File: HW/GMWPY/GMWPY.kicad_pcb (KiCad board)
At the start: 4 copper layers, 77.6 x 33.4 mm, 63 parts, among them J1 USB_C_Receptacle, J2 Micro_SD_Card_Det, Q1 Q_PJFET_DSG, U1 AMS1117-3.3, U10 LM4040DBZ-2.0, U11 ESP32-S3-WROOM-1, U2 SRV05-4, U3 USEQGCDACH4100, U4 TSV991ILT, U5 TSV991ILT, U6 TSV991ILT, U7 TSV991ILT, U8 TSV991ILT, U9 TSV991ILT

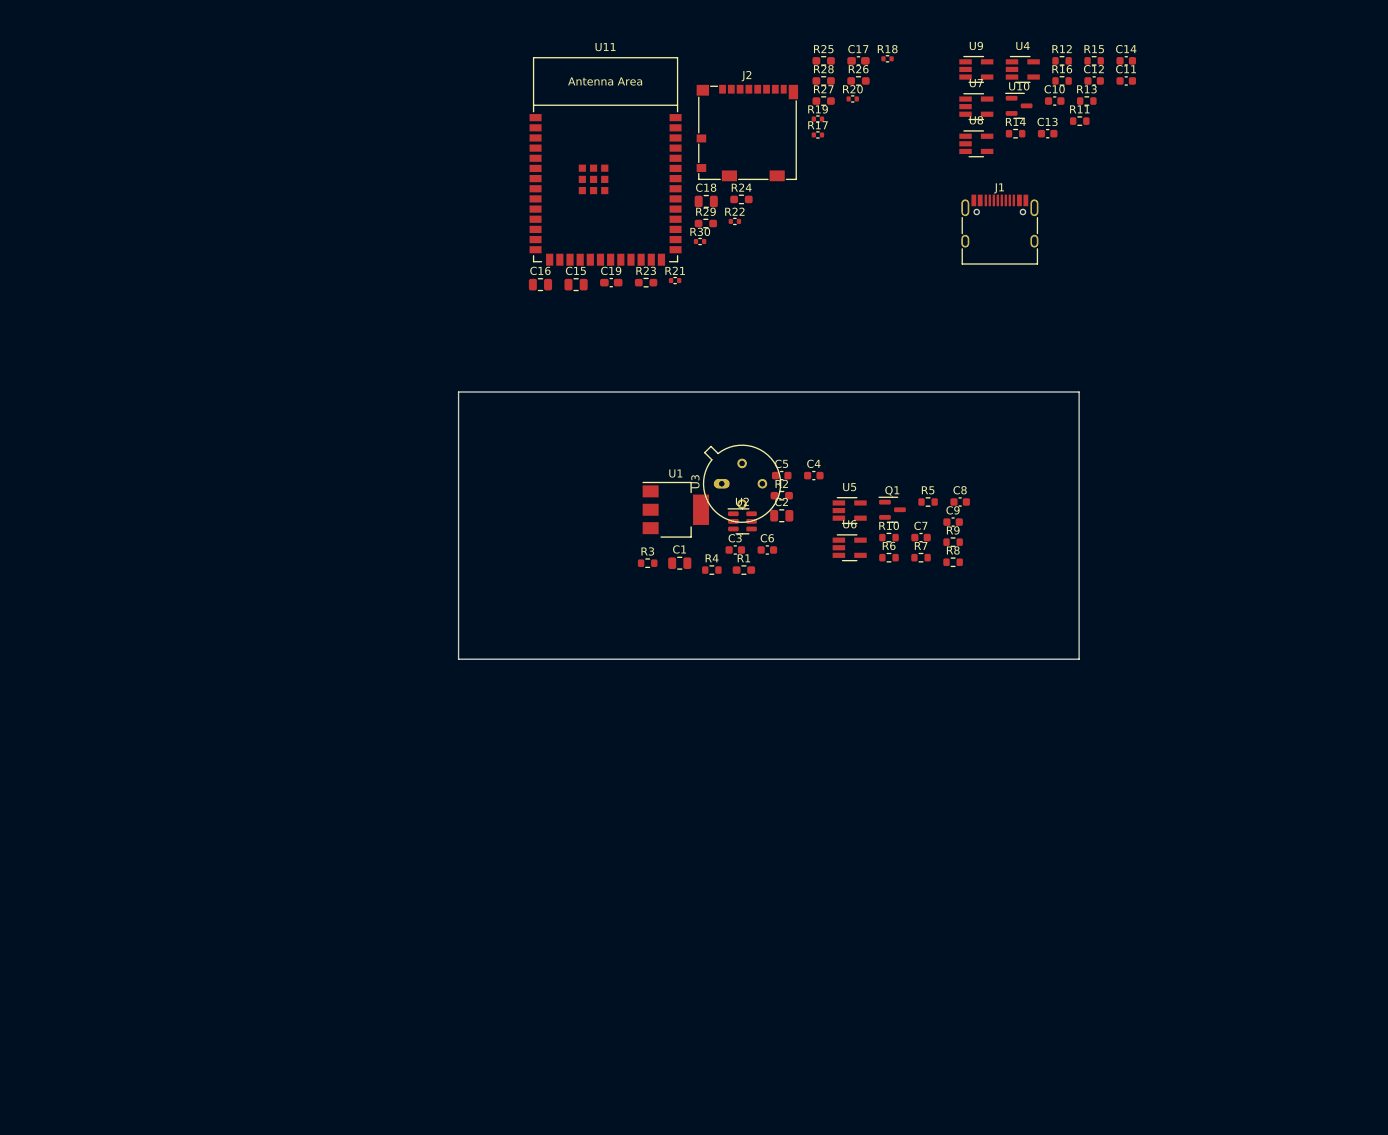
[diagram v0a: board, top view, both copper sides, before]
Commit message: G
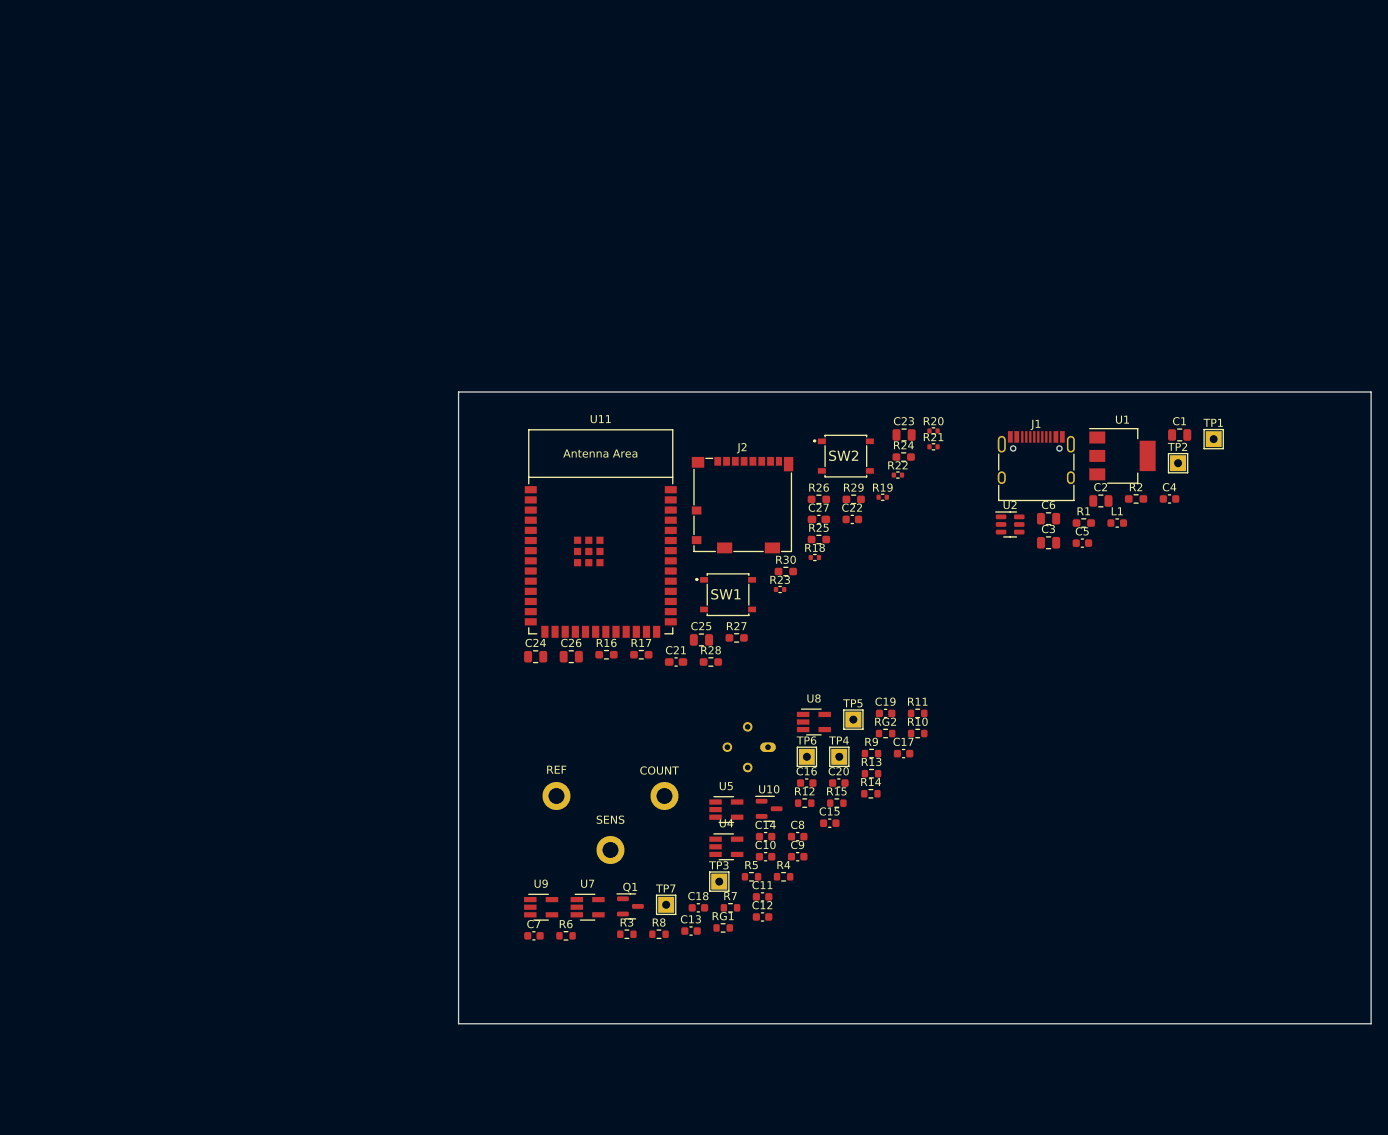
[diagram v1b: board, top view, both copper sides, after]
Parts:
- added C20: 2u2, Capacitor_SMD:C_0603_1608Metric, F.Cu at (131.8, 132.5)
- added C21: 100n, Capacitor_SMD:C_0603_1608Metric_Pad1.08x0.95mm_HandSolder, F.Cu at (111.4, 117.3)
- added C22: 2u2, Capacitor_SMD:C_0603_1608Metric, F.Cu at (133.4, 99.5)
- added C23: 10u, Capacitor_SMD:C_0805_2012Metric, F.Cu at (139.9, 89.0)
- added C24: 10u, Capacitor_SMD:C_0805_2012Metric, F.Cu at (93.9, 116.7)
- added C25: 10u, Capacitor_SMD:C_0805_2012Metric, F.Cu at (114.6, 114.6)
- added C26: 10u, Capacitor_SMD:C_0805_2012Metric, F.Cu at (98.3, 116.7)
- added C27: 100n, Capacitor_SMD:C_0603_1608Metric_Pad1.08x0.95mm_HandSolder, F.Cu at (129.3, 99.5)
- added L1: L_Small, Inductor_SMD:L_0603_1608Metric, F.Cu at (166.6, 100.0)
- added RG1: gain, Resistor_SMD:R_0603_1608Metric, F.Cu at (117.3, 150.6)
- added RG2: gain, Resistor_SMD:R_0603_1608Metric, F.Cu at (137.6, 126.3)
- added SW1: MCU_RESET, SamacSys_Parts:PTS526SK15SMTR2LFS, F.Cu at (117.9, 108.9)
- added SW2: MCU_RESET, SamacSys_Parts:PTS526SK15SMTR2LFS, F.Cu at (132.6, 91.6)
- added TP1: TestPoint, TestPoint:TestPoint_THTPad_2.0x2.0mm_Drill1.0mm, F.Cu at (178.6, 89.5)
- added TP2: TestPoint, TestPoint:TestPoint_THTPad_2.0x2.0mm_Drill1.0mm, F.Cu at (174.2, 92.5)
- added TP3: TestPoint, TestPoint:TestPoint_THTPad_2.0x2.0mm_Drill1.0mm, F.Cu at (116.8, 144.8)
- added TP4: TestPoint, TestPoint:TestPoint_THTPad_2.0x2.0mm_Drill1.0mm, F.Cu at (131.8, 129.2)
- added TP5: TestPoint, TestPoint:TestPoint_THTPad_2.0x2.0mm_Drill1.0mm, F.Cu at (133.6, 124.5)
- added TP6: TestPoint, TestPoint:TestPoint_THTPad_2.0x2.0mm_Drill1.0mm, F.Cu at (127.8, 129.2)
- added TP7: TestPoint, TestPoint:TestPoint_THTPad_2.0x2.0mm_Drill1.0mm, F.Cu at (110.2, 147.7)
- C10, C9: value 100n -> 2u2
- C12, C14: value 2u2 -> 3n3
- C15, C16: value 10u -> 100n; footprint Capacitor_SMD:C_0805_2012Metric -> Capacitor_SMD:C_0603_1608Metric
- C17, C19: value 100n -> 2u2; footprint Capacitor_SMD:C_0603_1608Metric_Pad1.08x0.95mm_HandSolder -> Capacitor_SMD:C_0603_1608Metric
- C18: value 10u -> 2u2; footprint Capacitor_SMD:C_0805_2012Metric -> Capacitor_SMD:C_0603_1608Metric
- C3: value 2u2 -> 10u; footprint Capacitor_SMD:C_0603_1608Metric -> Capacitor_SMD:C_0805_2012Metric
- C6: value 3n3 -> 10u; footprint Capacitor_SMD:C_0603_1608Metric -> Capacitor_SMD:C_0805_2012Metric
- C8: value 3n3 -> 2u2
- R10: value 10k -> 10
- R12: value 10 -> 10k
- R13: value 10k -> 1k
- R16: value 1k -> 10k; footprint Resistor_SMD:R_0603_1608Metric -> Resistor_SMD:R_0603_1608Metric_Pad0.98x0.95mm_HandSolder
- R17, R30: value 10 -> 10k; footprint Resistor_SMD:R_0402_1005Metric -> Resistor_SMD:R_0603_1608Metric_Pad0.98x0.95mm_HandSolder
- R23: value 10k -> 10; footprint Resistor_SMD:R_0603_1608Metric_Pad0.98x0.95mm_HandSolder -> Resistor_SMD:R_0402_1005Metric
- R7: value gain -> 1Meg
- R8: value 1Meg -> 10k
- U3: moved to B.Cu
- U6: value TSV991ILT -> EC4-1000-H2; footprint Package_TO_SOT_SMD:SOT-23-5_HandSoldering -> Z_mycustom_footprint_lib:EC4-3pin; moved to B.Cu
- moved U9 118.0 mm to (94.5, 148.0)
- moved C12 112.4 mm to (122.2, 149.2)
- moved C11 111.7 mm to (122.2, 146.7)
- moved U7 111.2 mm to (100.3, 148.0)
- moved C13 109.2 mm to (113.3, 151.0)
- moved C14 106.9 mm to (122.6, 139.2)
- moved U4 104.0 mm to (117.7, 140.4)
- moved C10 101.1 mm to (122.6, 141.7)
- moved R12 98.2 mm to (127.5, 135.0)
- moved R15 98.2 mm to (131.5, 135.0)
- moved U10 93.3 mm to (123.0, 135.7)
- moved R16 91.6 mm to (102.7, 116.4)
- moved C18 88.3 mm to (114.2, 148.1)
- moved R13 88.3 mm to (135.8, 131.3)
- moved C17 86.8 mm to (139.8, 128.8)
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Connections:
- net /Measurements/Gas renamed /GAS_Measurements/CH4_Gas
- net /Measurements/Ref renamed /GAS_Measurements/CH4_Ref
- C1 pad 1: +5V -> Net-(C1-Pad1)
- C10 pad 1: Net-(C10-Pad1) -> GND
- C10 pad 2: Net-(C10-Pad2) -> +5V
- C11 pad 2: +5V -> Net-(C11-Pad2)
- C12 pad 1: GND -> /GAS_Measurements/OUT2
- C12 pad 2: +5V -> /GAS_Measurements/CH4_V-ref
- C13 pad 2: +5V -> Net-(C13-Pad2)
- C14 pad 1: GND -> /GAS_Measurements/OUT1
- C14 pad 2: Net-(C14-Pad2) -> /GAS_Measurements/CH4_V-gas
- C15 pad 1: +3V3 -> /GAS_Measurements/OUT3
- C15 pad 2: GND -> /GAS_Measurements/H2_V-
- C16 pad 1: +3V3 -> /GAS_Measurements/H2_counter
- C16 pad 2: GND -> Net-(C16-Pad2)
- C17 pad 1: +3V3 -> GND
- C17 pad 2: GND -> +5V
- C18 pad 1: +3V3 -> GND
- C18 pad 2: GND -> +5V
- C19 pad 1: +3V3 -> GND
- C19 pad 2: GND -> +5V
- C3 pad 1: GND -> Net-(C1-Pad1)
- C3 pad 2: +5V -> GND
- C4 pad 2: +5V -> Net-(C1-Pad1)
- C5 pad 2: Net-(C5-Pad2) -> +5V
- C6 pad 1: /Measurements/OUT2 -> +5V
- C6 pad 2: /Measurements/V-ref -> GND
- C7 pad 2: Net-(C7-Pad2) -> +5V
- C8 pad 1: /Measurements/OUT1 -> GND
- C8 pad 2: /Measurements/V-gas -> +5V
- C9 pad 1: /Measurements/OUT3 -> GND
- C9 pad 2: Net-(C9-Pad2) -> +5V
- J2 pad 10: /MCU/CARD_DETECT -> GPIO_40
- Q1 pad 1: Net-(Q1-Pad1) -> /GAS_Measurements/H2_reference
- Q1 pad 2: Net-(Q1-Pad2) -> /GAS_Measurements/H2_sensing
- R10 pad 1: Net-(Q1-Pad1) -> /GAS_Measurements/H2_V-
- R10 pad 2: Net-(C10-Pad2) -> /GAS_Measurements/H2_sensing
- R11 pad 1: Net-(C9-Pad2) -> REF
- R11 pad 2: Net-(Q1-Pad2) -> /GAS_Measurements/H2_V+
- R12 pad 1: REF -> Net-(R12-Pad1)
- R12 pad 2: Net-(R12-Pad2) -> REF
- R13 pad 1: Net-(R13-Pad1) -> +5V
- R13 pad 2: REF -> 2V048
- R14 pad 1: +5V -> /GAS_Measurements/1V012
- R14 pad 2: Net-(C14-Pad2) -> 2V048
- R15 pad 1: Net-(R15-Pad1) -> /GAS_Measurements/1V012
- R15 pad 2: Net-(C14-Pad2) -> GND
- R16 pad 1: Net-(R15-Pad1) -> +3V3
- R16 pad 2: GND -> /MCU/ESP_EN
- R17 pad 1: /MCU/DATA_0 -> /MCU/ESP_BOOT
- R17 pad 2: GPIO_42 -> +3V3
- R18 pad 1: /MCU/DATA_1 -> /MCU/DATA_0
- R18 pad 2: GPIO_41 -> GPIO_42
- R19 pad 1: /MCU/DATA_2 -> /MCU/DATA_1
- R19 pad 2: GPIO_1 -> GPIO_41
- R20 pad 1: /MCU/DATA_3 -> /MCU/DATA_2
- R20 pad 2: GPIO_2 -> GPIO_1
- R21 pad 1: /MCU/CMD -> /MCU/DATA_3
- R21 pad 2: GPIO_43 -> GPIO_2
- R22 pad 1: /MCU/CLK -> /MCU/CMD
- R22 pad 2: GPIO_44 -> GPIO_43
- R23 pad 1: /MCU/DATA_0 -> /MCU/CLK
- R23 pad 2: +3V3 -> GPIO_44
- R24 pad 1: /MCU/DATA_1 -> /MCU/DATA_0
- R25 pad 1: /MCU/DATA_2 -> /MCU/DATA_1
- R26 pad 1: /MCU/DATA_3 -> /MCU/DATA_2
- R27 pad 1: /MCU/CMD -> /MCU/DATA_3
- R28 pad 1: /MCU/CLK -> /MCU/CMD
- R29 pad 1: /MCU/CARD_DETECT -> /MCU/CLK
- R3 pad 1: Net-(C5-Pad2) -> Net-(C11-Pad2)
- R3 pad 2: /Measurements/V-ref -> /GAS_Measurements/CH4_V-ref
- R30 pad 1: /MCU/CARD_DETECT -> GPIO_40
- R30 pad 2: GPIO_40 -> +3V3
- R4 pad 1: Net-(C7-Pad2) -> Net-(C13-Pad2)
- R4 pad 2: /Measurements/V-gas -> /GAS_Measurements/CH4_V-gas
- R5 pad 1: /Measurements/OUT2 -> /GAS_Measurements/OUT2
- R5 pad 2: /Measurements/V-ref -> /GAS_Measurements/CH4_V-ref
- R6 pad 1: /Measurements/OUT1 -> /GAS_Measurements/OUT1
- R6 pad 2: /Measurements/V-gas -> /GAS_Measurements/CH4_V-gas
- R7 pad 1: /Measurements/OUT3 -> GND
- R7 pad 2: Net-(C9-Pad2) -> Net-(Q1-Pad3)
- R8 pad 1: GND -> Net-(C16-Pad2)
- R8 pad 2: Net-(Q1-Pad3) -> Net-(R8-Pad2)
- R9 pad 1: Net-(C10-Pad2) -> /GAS_Measurements/H2_reference
- R9 pad 2: Net-(R9-Pad2) -> Net-(C16-Pad2)
- U1 pad 3: +5V -> Net-(C1-Pad1)
- U10 pad 1: Net-(C14-Pad2) -> 2V048
- U4 pad 1: /Measurements/OUT2 -> /GAS_Measurements/OUT2
- U4 pad 4: /Measurements/V-ref -> /GAS_Measurements/CH4_V-ref
- U5 pad 1: /Measurements/OUT1 -> /GAS_Measurements/OUT1
- U5 pad 4: /Measurements/V-gas -> /GAS_Measurements/CH4_V-gas
- U6 pad 1: Net-(U4-Pad3) -> /GAS_Measurements/H2_reference
- U6 pad 2: GND -> /GAS_Measurements/H2_sensing
- U6 pad 3: Net-(R10-Pad1) -> /GAS_Measurements/H2_counter
- U7 pad 1: /Measurements/OUT3 -> /GAS_Measurements/OUT3
- U7 pad 3: Net-(R12-Pad2) -> /GAS_Measurements/H2_V+
- U7 pad 4: Net-(C9-Pad2) -> /GAS_Measurements/H2_V-
- U8 pad 1: Net-(C10-Pad1) -> /GAS_Measurements/H2_counter
- U8 pad 3: Net-(R13-Pad1) -> Net-(R12-Pad1)
- U8 pad 4: Net-(R9-Pad2) -> Net-(R8-Pad2)
- U9 pad 3: Net-(R15-Pad1) -> /GAS_Measurements/1V012
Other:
- board size 77.6 x 33.4 mm -> 114.1 x 79 mm

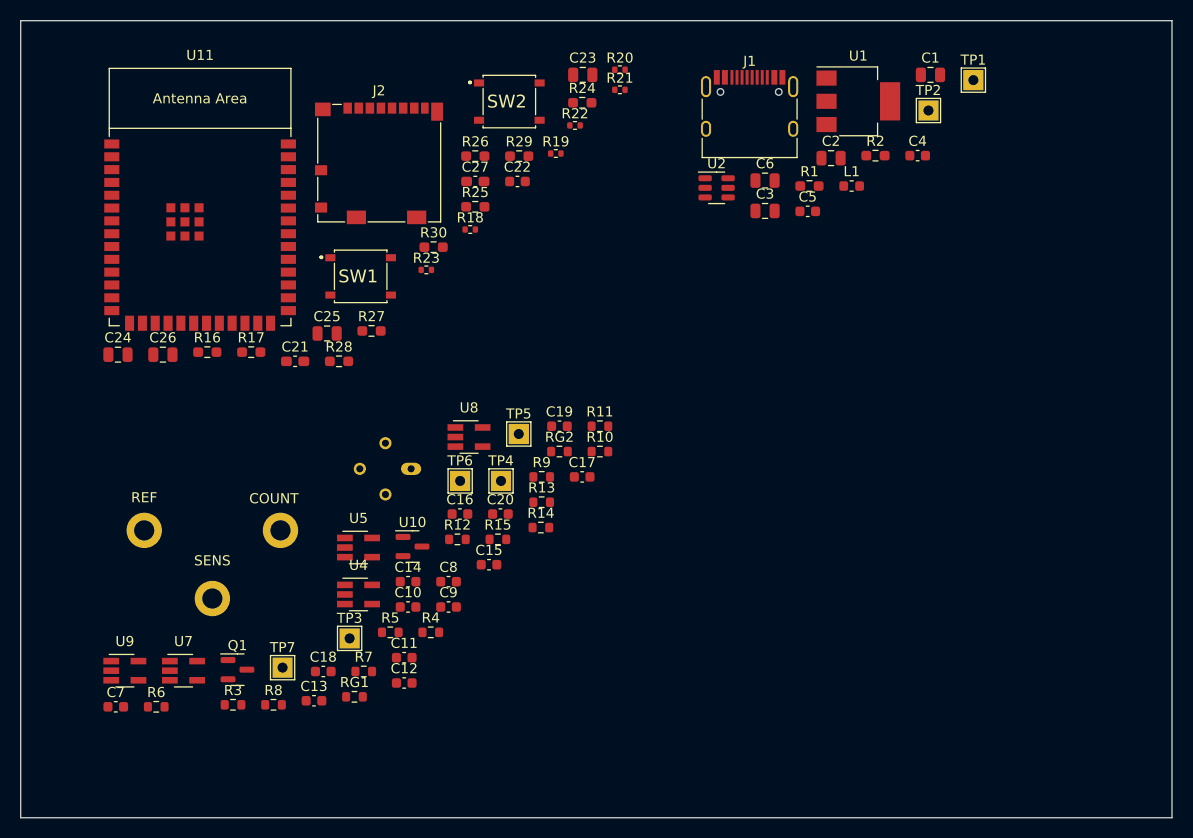
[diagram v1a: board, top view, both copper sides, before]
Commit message: t
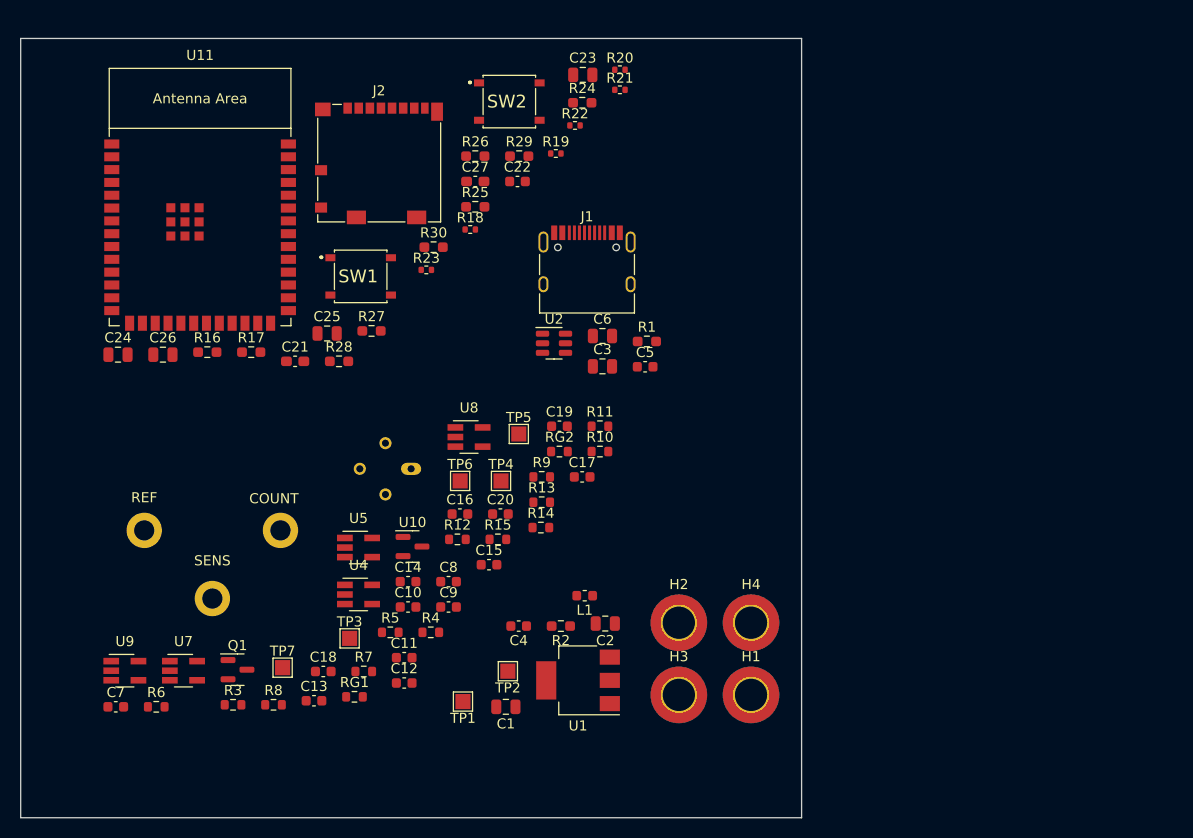
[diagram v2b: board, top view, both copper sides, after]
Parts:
- added H1: MountingHole_Pad, MountingHole:MountingHole_3.2mm_M3_DIN965_Pad_TopBottom, F.Cu at (156.6, 150.4)
- added H2: MountingHole_Pad, MountingHole:MountingHole_3.2mm_M3_DIN965_Pad_TopBottom, F.Cu at (149.4, 143.2)
- added H3: MountingHole_Pad, MountingHole:MountingHole_3.2mm_M3_DIN965_Pad_TopBottom, F.Cu at (149.4, 150.4)
- added H4: MountingHole_Pad, MountingHole:MountingHole_3.2mm_M3_DIN965_Pad_TopBottom, F.Cu at (156.6, 143.2)
- TP1, TP2, TP3, TP4, TP5, TP6, TP7: footprint TestPoint:TestPoint_THTPad_2.0x2.0mm_Drill1.0mm -> TestPoint:TestPoint_Pad_1.5x1.5mm
- moved TP1 79.7 mm to (128.0, 151.1), turned to 180 degrees
- moved C1 75.4 mm to (132.3, 151.6), turned to 180 degrees
- moved TP2 69.4 mm to (132.5, 148.1), turned to 180 degrees
- moved U1 63.7 mm to (139.4, 149.0), turned to 180 degrees
- moved C4 61.1 mm to (133.6, 143.6), turned to 180 degrees
- moved R2 56.1 mm to (137.7, 143.6), turned to 180 degrees
- moved C2 51.2 mm to (142.1, 143.3), turned to 180 degrees
- moved L1 48.4 mm to (140.1, 140.6), turned to 180 degrees
- moved R1 22.3 mm to (146.3, 115.4)
- moved C5 22.3 mm to (146.1, 117.9)
- moved C6 22.3 mm to (141.9, 114.8)
- moved U2 22.3 mm to (137.1, 115.6)
- moved C3 22.3 mm to (141.9, 117.8)
- moved J1 22.3 mm to (140.3, 108.7)
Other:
- board size 114.1 x 79 mm -> 77.4 x 77.2 mm
